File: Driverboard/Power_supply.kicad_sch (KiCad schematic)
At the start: 61 parts, among them IC1 INA226AQDGSRQ1, IC2 LTC2955CTS8-1#TRMPBF, IC3 LTC4415EMSE#PBF, IC4 LMR23630ADDA, IC5 LT3080IST#WPBF, IC6 LMR23630ADDA, Q1 FDD86367, U1 LTC4231CMS-2-PBF

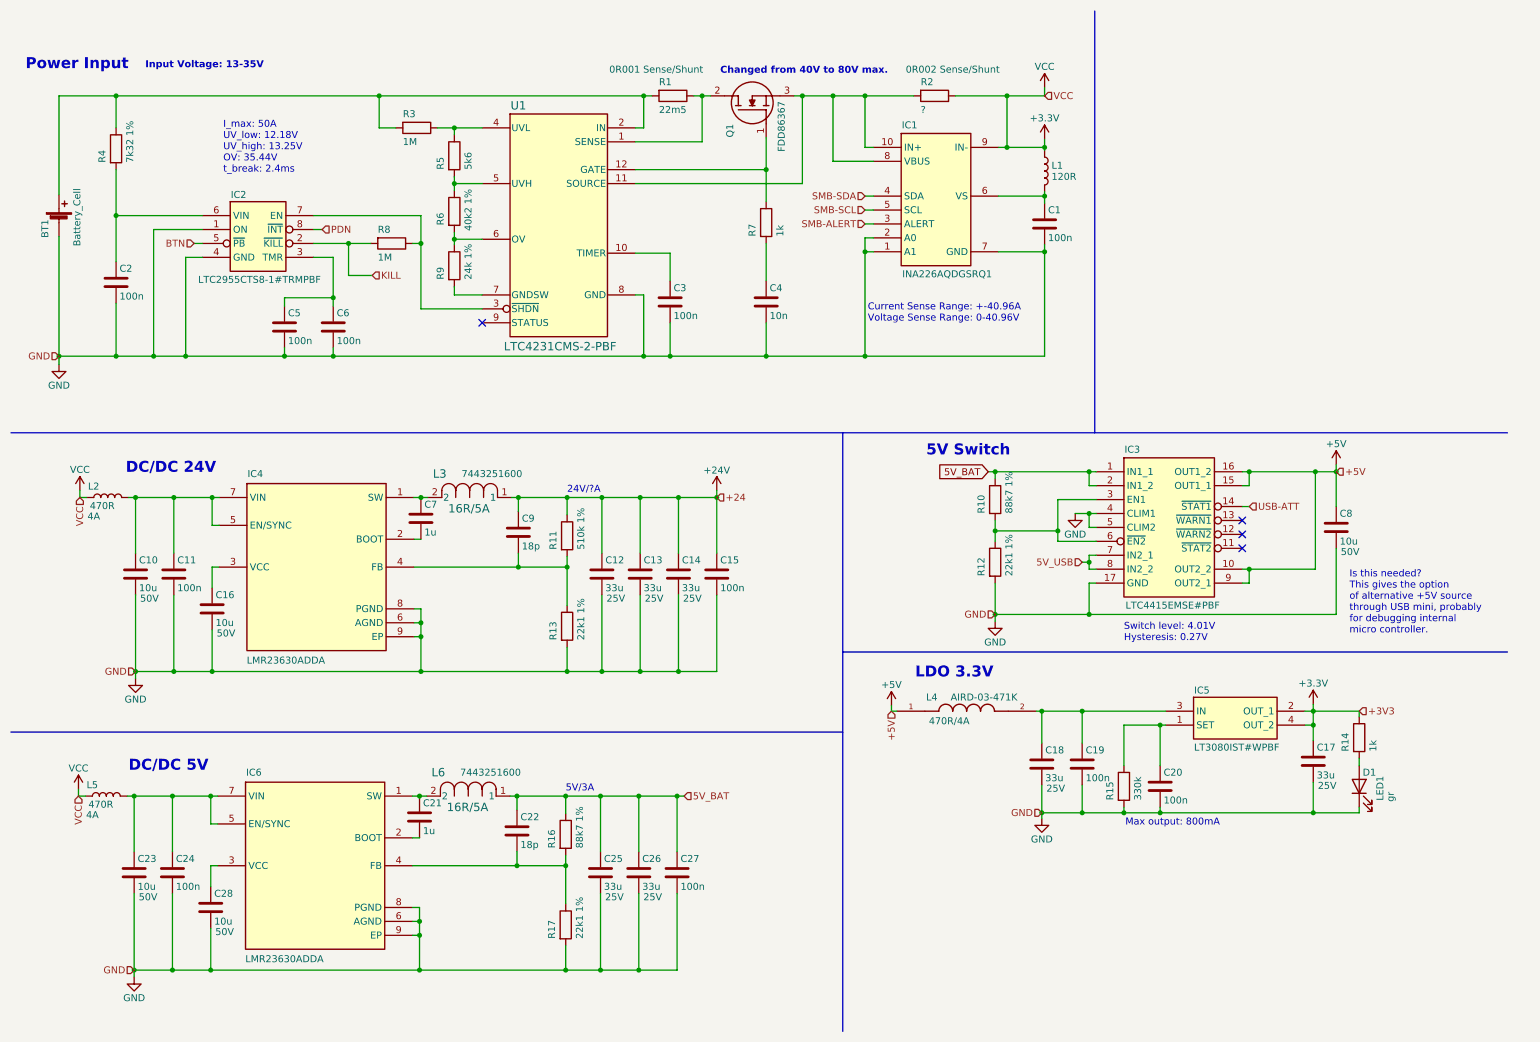
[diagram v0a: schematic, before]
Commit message: WIP
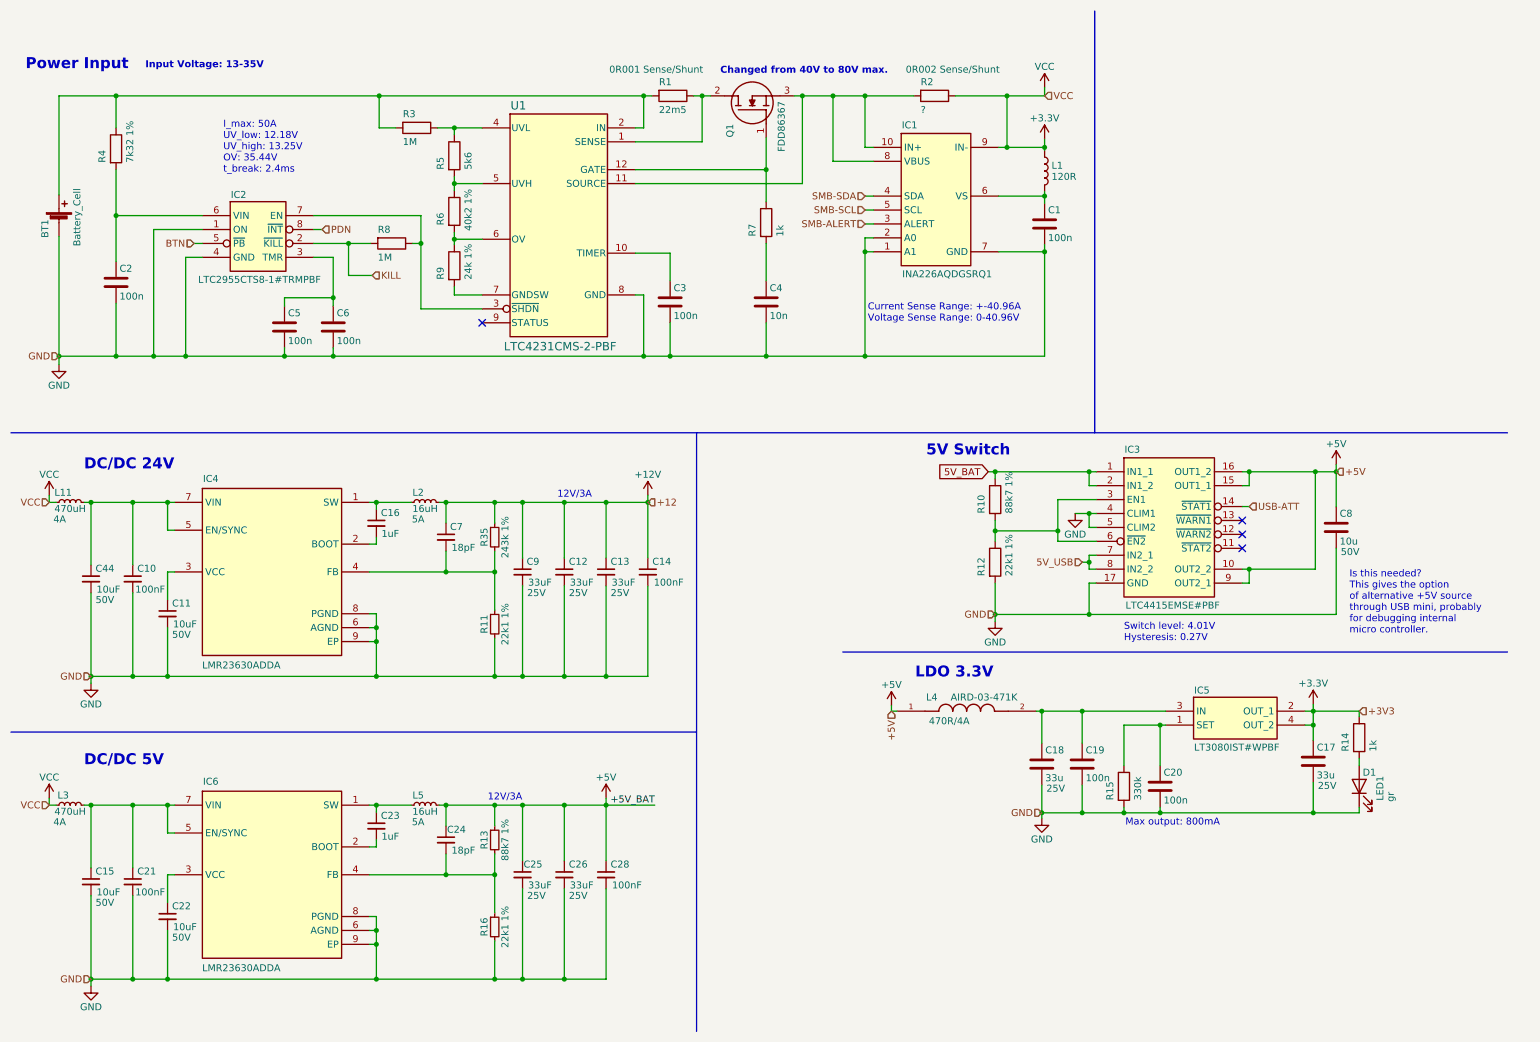
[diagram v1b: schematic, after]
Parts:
- removed C10, C16, C23, C28: 10u, symbol Device:C
- removed C11, C15, C24, C27: 100n, symbol Device:C
- removed C12, C13, C14, C25, C26: 33u, symbol Device:C
- removed C21, C7: 1u, symbol Device:C
- removed C22, C9: 18p, symbol Device:C
- removed L2, L5: 470R, symbol Device:L
- removed L3, L6: 16R/5A, IND_1050-WE-HCI_WRE, symbol CustomSymbols:7443251600
- removed R11: 510k 1%, symbol Device:R
- removed R13, R17: 22k1 1%, symbol Device:R
- removed R16: 88k7 1%, symbol Device:R
- added C10, C14, C21, C28: 100nF, symbol Device:C_Small
- added C11, C15, C22, C44: 10uF, symbol Device:C_Small
- added C12, C13, C25, C26, C9: 33uF, symbol Device:C_Small
- added C16, C23: 1uF, symbol Device:C_Small
- added C24, C7: 18pF, symbol Device:C_Small
- added L11, L3: 470uH, symbol Device:L_Small
- added L2, L5: 16uH, symbol Device:L_Small
- added R11, R16: 22k1 1%, symbol Device:R_Small
- added R13: 88k7 1%, symbol Device:R_Small
- added R35: 243k 1%, symbol Device:R_Small
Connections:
- net +3.3V: now also L11.1, L3.1
- net +5V: now also C24.1, C25.1, C26.1, C28.1, L5.2, R13.1
- net GND: now also C10.2, C11.2, C12.2, C13.2, C14.2, C15.2, C21.2, C22.2, C25.2, C26.2, C28.2, C44.2, C9.2, R11.2, R16.2
- net at IC4.3 (VCC): now also C11.1
- net at IC6.4 (FB): now also C24.2, R13.2, R16.1
- net at IC6.5 (EN/SYNC), IC6.7 (VIN): now also C15.1, C21.1, L3.2
- net at IC6.1 (SW): now also C23.1, L5.1
- net at IC4.5 (EN/SYNC), IC4.7 (VIN): now also C10.1, C44.1, L11.2
- net at IC4.4 (FB): now also C7.2, R11.1, R35.2
- net at IC4.1 (SW): now also C16.1, L2.1
- net at IC4.2 (BOOT): now also C16.2
- net at IC6.2 (BOOT): now also C23.2
- net at IC6.3 (VCC): now also C22.1
- new net +12V: C12.1, C13.1, C14.1, C7.1, C9.1, L2.2, R35.1
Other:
- note added: "12V/3A"
- note removed: "24V/?A"
- note removed: "5V/3A"
- moved on the sheet: IC4
